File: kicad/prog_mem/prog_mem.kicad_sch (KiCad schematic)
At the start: 36 parts

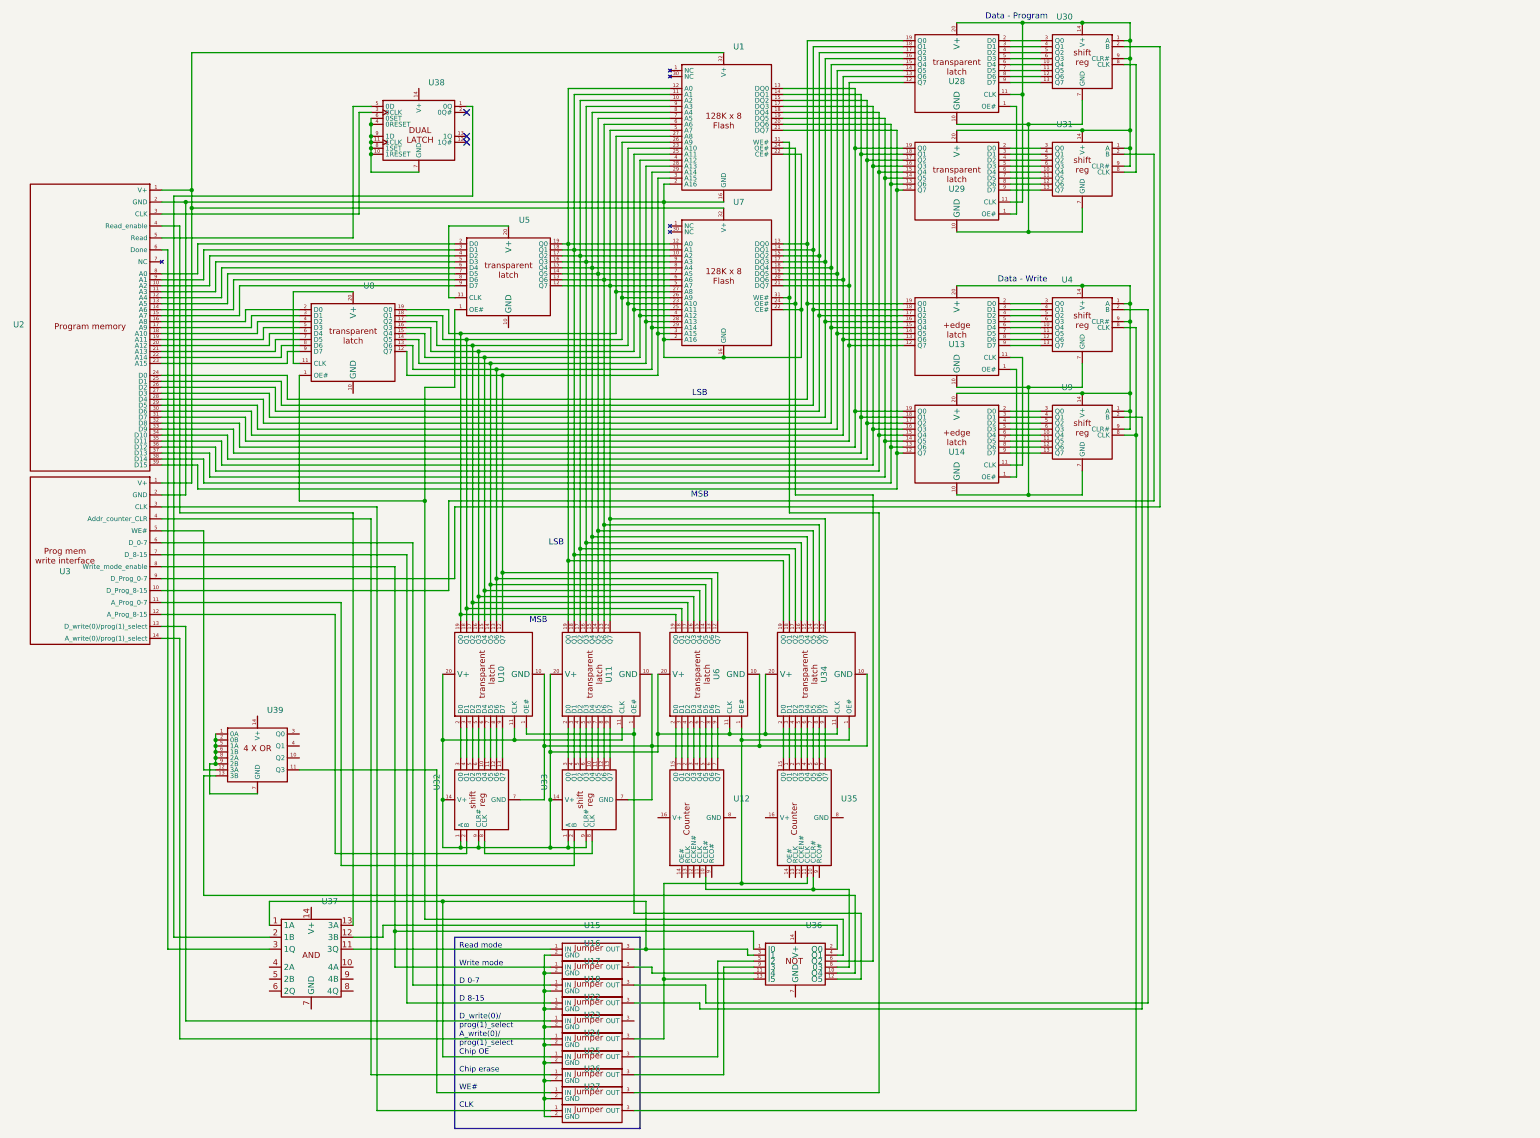
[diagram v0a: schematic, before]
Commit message: Finished prog mem schematic
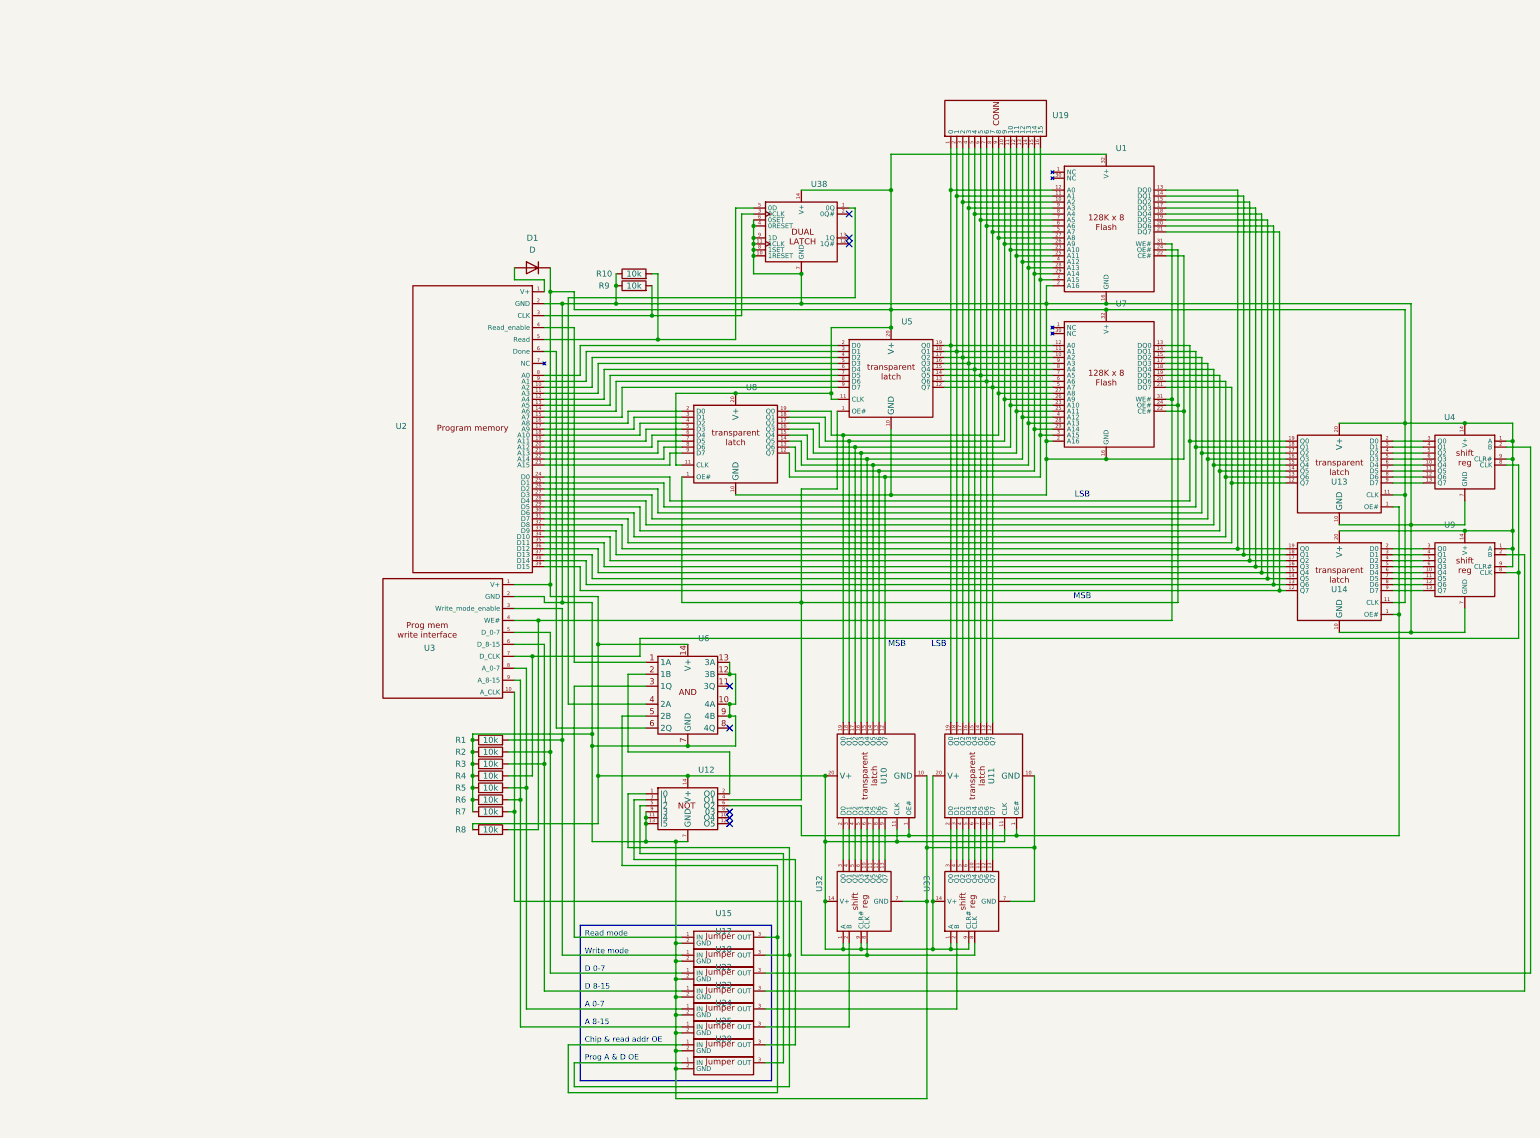
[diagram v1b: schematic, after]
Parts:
- removed U12, U35: ~, Package_DIP:DIP-16_W7.62mm, symbol custom_symbol_lib:8_bit_counter
- removed U16, U26, U27: ~, custom_footprint_library:jumper, symbol custom_symbol_lib:jumper
- removed U28, U29, U34, U6: ~, Package_DIP:DIP-20_W7.62mm, symbol custom_symbol_lib:8_bit_transparent_latch
- removed U30, U31: ~, Package_DIP:DIP-14_W7.62mm, symbol custom_symbol_lib:8_bit_shift_register
- removed U36: ~, Package_DIP:DIP-14_W7.62mm, symbol custom_symbol_lib:6xNOT
- removed U37: ~, Package_DIP:DIP-14_W7.62mm, symbol custom_symbol_lib:quad_and
- removed U39: ~, Package_DIP:DIP-14_W7.62mm, symbol custom_symbol_lib:quad_OR
- added D1: D, Diode_THT:D_A-405_P7.62mm_Horizontal, symbol Device:D
- added R1, R10, R2, R3, R4, R5, R6, R7, R8, R9: 10k, custom_footprint_library:0.4_pitch_resistor, symbol Device:R
- added U12: ~, Package_DIP:DIP-14_W7.62mm, symbol custom_symbol_lib:6xNOT
- added U19: ~, Connector_PinHeader_2.54mm:PinHeader_1x16_P2.54mm_Vertical, symbol custom_symbol_lib:connector_16_bit
- added U20: ~, custom_footprint_library:jumper, symbol custom_symbol_lib:jumper
- added U6: ~, Package_DIP:DIP-14_W7.62mm, symbol custom_symbol_lib:quad_and
- U13, U14: symbol custom_symbol_lib:rising_edge_8_bit_latch -> custom_symbol_lib:8_bit_transparent_latch
- U3: footprint Connector_PinHeader_2.54mm:PinHeader_1x08_P2.54mm_Horizontal -> Connector_PinHeader_2.54mm:PinHeader_1x10_P2.54mm_Horizontal
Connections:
- net at U18.1 (IN): now also U3.5 (D_0-7), R2.2; no longer U3.7 (D_8-15)
- net at U15.2 (GND), U17.2 (GND), U18.2 (GND)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: now also U1.16 (GND), U1.2 (A16), U1.22 (CE#), U10.10 (GND), U11.10 (GND), U13.10 (GND), U14.10 (GND), U2.2 (GND), U3.2 (GND), U32.7 (GND), U33.7 (GND), U38.10 (1RESET), U38.11 (1CLK), U38.4 (0RESET), U38.6 (0SET), U38.7 (GND), U38.8 (1SET), U38.9 (1D), U4.7 (GND), U5.10 (GND), U7.16 (GND), U7.2 (A16), U7.22 (CE#), U8.10 (GND), U9.7 (GND), R1.1, R10.1, R2.1, R3.1, R4.1, R5.1, R6.1, R7.1, R9.1, U12.11 (I4), U12.13 (I5), U12.7 (GND), U12.9 (I3), U20.2 (GND), U6.10 (4A), U6.12 (3B), U6.13 (3A), U6.7 (GND), U6.9 (4B)
- net at U18.3 (OUT): now also U4.2 (B); no longer U9.2 (B)
- net at U23.3 (OUT): now also U33.2 (B)
- net at U10.11 (CLK), U10.20 (V+), U11.11 (CLK)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: now also U1.32 (V+), U13.11 (CLK), U13.20 (V+), U14.11 (CLK), U14.20 (V+), U3.1 (V+), U38.14 (V+), U4.1 (A), U4.14 (V+), U4.9 (CLR#), U5.11 (CLK), U5.20 (V+), U7.32 (V+), U8.11 (CLK), U8.20 (V+), U9.1 (A), U9.14 (V+), U9.9 (CLR#), D1.1 (K), R8.1, U12.14 (V+), U6.14 (V+)
- net at U1.5 (A7), U11.12 (Q7), U5.12 (Q7)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: now also U19.8 (7)
- net at U1.6 (A6), U11.13 (Q6), U5.13 (Q6)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: now also U19.7 (6)
- net at U1.7 (A5), U11.14 (Q5), U5.14 (Q5)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: now also U19.6 (5)
- net at U1.8 (A4), U11.15 (Q4), U5.15 (Q4)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: now also U19.5 (4)
- net at U1.9 (A3), U11.16 (Q3), U5.16 (Q3)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: now also U19.4 (3)
- net at U1.10 (A2), U11.17 (Q2), U5.17 (Q2)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: now also U19.3 (2)
- net at U1.11 (A1), U11.18 (Q1), U5.18 (Q1)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: now also U19.2 (1)
- net at U1.12 (A0), U11.19 (Q0), U5.19 (Q0)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: now also U19.1 (0)
- net at U25.1 (IN): now also U15.3 (OUT), U6.5 (2B); no longer U3.4 (Addr_counter_CLR)
- net at U25.3 (OUT): now also U12.3 (I1)
- net at U38.1 (0Q): now also U6.4 (2A)
- net at U2.3 (CLK), U38.3 (0CLK): now also R9.2
- net at U2.5 (Read), U38.5 (0D): now also R10.2
- net at U22.1 (IN): now also U3.6 (D_8-15), R3.2; no longer U3.13 (D_write(0)/prog(1)_select)
- net at U22.3 (OUT): now also U9.2 (B)
- net at U15.1 (IN): now also U6.3 (1Q)
- net at U24.1 (IN): now also U3.9 (A_8-15), R6.2; no longer U15.3 (OUT)
- net at U3.3 (Write_mode_enable): now also U17.1 (IN), R1.2
- net at U4.8 (CLK), U9.8 (CLK): now also U3.7 (D_CLK), R4.2
- net at U3.8 (A_0-7): now also U23.1 (IN), R5.2
- net at U10.1 (OE#), U11.1 (OE#): now also U13.1 (OE#), U14.1 (OE#), U12.6 (O2)
- net at U5.1 (OE#), U8.1 (OE#): now also U1.24 (OE#), U7.24 (OE#), U12.4 (O1)
- net at U24.3 (OUT): now also U32.2 (B)
- net at U3.10 (A_CLK): now also U32.8 (CLK), U33.8 (CLK), R7.2
- net at U1.23 (A10), U10.17 (Q2), U7.23 (A10)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: now also U19.11 (10)
- net at U1.25 (A11), U10.16 (Q3), U7.25 (A11)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: now also U19.12 (11)
- net at U1.26 (A9), U10.18 (Q1), U7.26 (A9)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: now also U19.10 (9)
- net at U1.27 (A8), U10.19 (Q0), U7.27 (A8)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: now also U19.9 (8)
- net at U1.28 (A13), U10.14 (Q5), U7.28 (A13)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: now also U19.14 (13)
- net at U1.29 (A14), U10.13 (Q6), U7.29 (A14)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: now also U19.15 (14)
- net at U1.3 (A15), U10.12 (Q7), U7.3 (A15)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: now also U19.16 (15)
- net at U1.31 (WE#), U7.31 (WE#): now also U3.4 (WE#), R8.2
- net at U1.4 (A12), U10.15 (Q4), U7.4 (A12)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: now also U19.13 (12)
- net at U2.4 (Read_enable): now also U6.1 (1A)
- net at U2.6 (Done): now also U6.6 (2Q)
- net at U17.3 (OUT): now also U12.1 (I0), U20.1 (IN); no longer U4.2 (B)
- new net: U12.2 (O0), U6.2 (1B)
- new net: U12.5 (I2), U20.3 (OUT)
- new net: D1.2 (A), U2.1 (V+)
- no-connect marks 3 -> 8
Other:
- note removed: "Data - Program"
- note removed: "Data - Write"
- moved on the sheet: U1, U10, U11, U13, U14, U15, U17, U18, U2, U22, U23, U24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
